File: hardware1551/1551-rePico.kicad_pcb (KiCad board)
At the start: 2 copper layers, 59.1 x 60 mm, 44 parts, among them IC1 VIA6522, J1 Display Connector, J2 Display Power, J3 Conn_01x05_Pin, J4 SD Card Module Connector, J5 Conn_01x01_Pin, J6 EXT_5V, J7 RESET_1541, P1 VIA_PIN_1-20, P2 VIA_PIN_21-40, Q1 BSS138, Q2 BSS138, Q3 BSS138, Q4 BSS138, Q5 BSS138, Q6 BSS138, Q7 BSS138, Q8 BSS138, Q9 BSS138, SW1 RESET, U1 Pico, U2 SN74LVC4245A

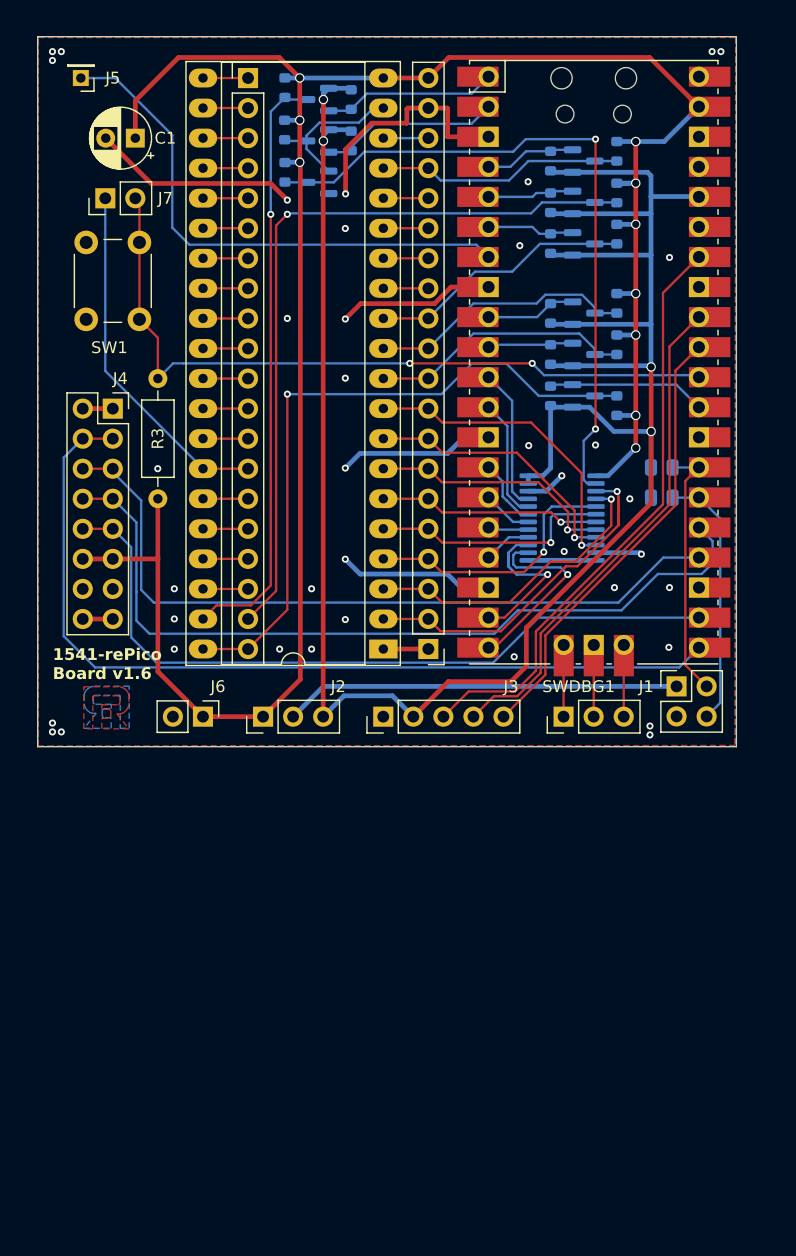
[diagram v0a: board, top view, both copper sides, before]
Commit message: updated
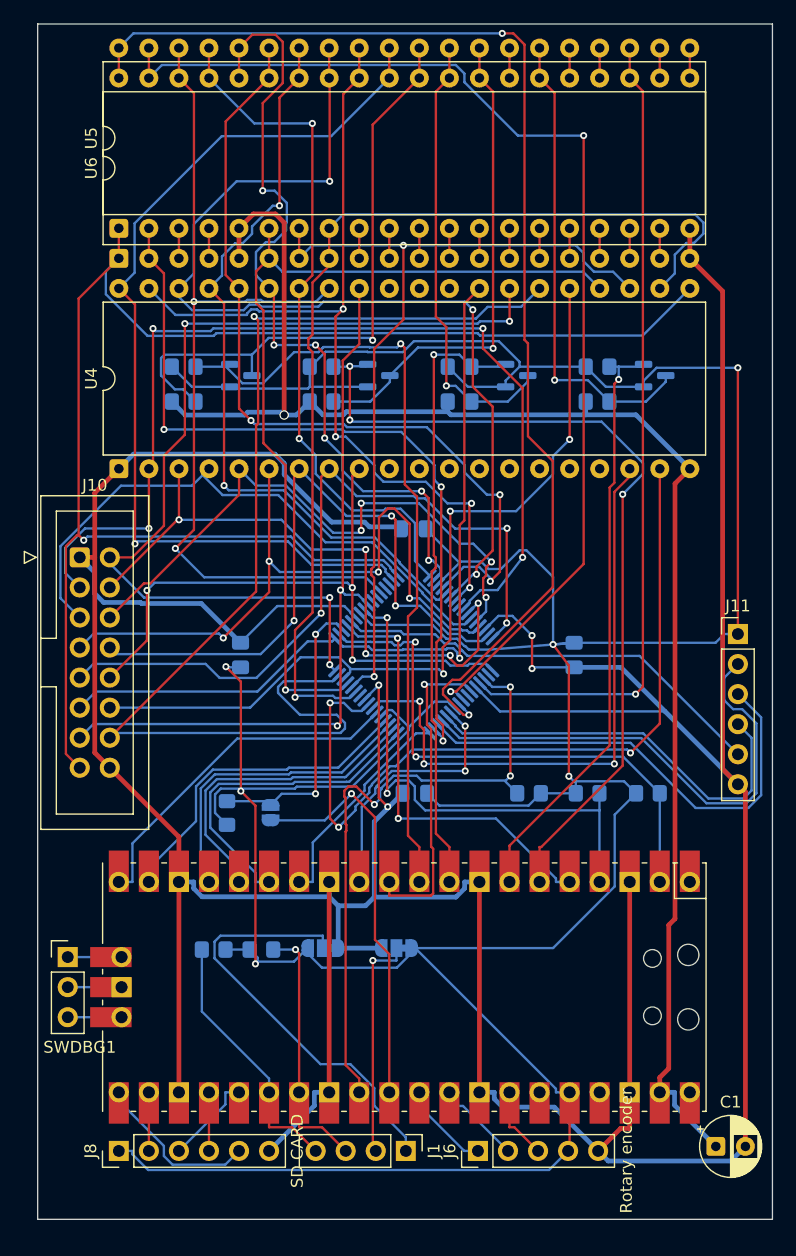
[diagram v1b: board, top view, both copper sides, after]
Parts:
- removed IC1: VIA6522, Package_DIP:DIP-40_W15.24mm_Socket_LongPads
- removed J2: Display Power, Connector_PinHeader_2.54mm:PinHeader_1x03_P2.54mm_Vertical
- removed J3: Conn_01x05_Pin, Connector_PinHeader_2.54mm:PinHeader_1x05_P2.54mm_Vertical
- removed J4: SD Card Module Connector, Connector_PinSocket_2.54mm:PinSocket_2x08_P2.54mm_Vertical
- removed J5: Conn_01x01_Pin, Connector_PinHeader_2.00mm:PinHeader_1x01_P2.00mm_Vertical
- removed J7: RESET_1541, Connector_PinHeader_2.54mm:PinHeader_1x02_P2.54mm_Vertical
- removed P1: VIA_PIN_1-20, Connector_PinHeader_2.54mm:PinHeader_1x20_P2.54mm_Vertical
- removed P2: VIA_PIN_21-40, Connector_PinHeader_2.54mm:PinHeader_1x20_P2.54mm_Vertical
- removed Q5, Q6, Q7, Q8, Q9: BSS138, Package_TO_SOT_SMD:SOT-23
- removed R15, R16, R17, R18, R19, R20: 10k, Resistor_SMD:R_0603_1608Metric
- removed SW1: RESET, Button_Switch_THT:SW_PUSH_6mm_H5mm
- removed U2: SN74LVC4245A, Package_SO:TSSOP-24_4.4x7.8mm_P0.65mm
- added C2: 0.1uF, Capacitor_SMD:C_0805_2012Metric_Pad1.18x1.45mm_HandSolder, B.Cu at (117.3, 117.3)
- added C3: 0.1uF, Capacitor_SMD:C_0805_2012Metric_Pad1.18x1.45mm_HandSolder, B.Cu at (145.5, 117.3)
- added C4: 0.1uF, Capacitor_SMD:C_0805_2012Metric_Pad1.18x1.45mm_HandSolder, B.Cu at (132.1, 129.0)
- added C5: 0.1uF, Capacitor_SMD:C_0805_2012Metric_Pad1.18x1.45mm_HandSolder, B.Cu at (131.9, 106.7)
- added J10: TCBM, Connector_IDC:IDC-Header_2x08_P2.54mm_Vertical, F.Cu at (103.7, 109.1)
- added J11: JTAG, Connector_PinHeader_2.54mm:PinHeader_1x06_P2.54mm_Vertical, F.Cu at (159.4, 115.5)
- added J8: SD CARD, Connector_PinHeader_2.54mm:PinHeader_1x06_P2.54mm_Vertical, F.Cu at (107.0, 159.2)
- added JP1: ~, Jumper:SolderJumper-2_P1.3mm_Open_RoundedPad1.0x1.5mm, B.Cu at (119.9, 130.6)
- added JP3: SolderJumper_3_Bridged12, Jumper:SolderJumper-3_P1.3mm_Bridged12_RoundedPad1.0x1.5mm_NumberLabels, B.Cu at (124.3, 142.1)
- added JP4: SolderJumper_3_Bridged12, Jumper:SolderJumper-3_P1.3mm_Bridged12_RoundedPad1.0x1.5mm_NumberLabels, B.Cu at (130.5, 142.1)
- added U3: XC9572XL-VQ64, Package_QFP:TQFP-64_10x10mm_P0.5mm, B.Cu at (132.0, 117.3)
- added U4: 6523 (pins), Package_DIP:DIP-40_W15.24mm, F.Cu at (107.0, 101.6)
- added U5: 6510T (pins), Package_DIP:DIP-40_W15.24mm, F.Cu at (107.0, 81.3)
- added U6: 6510T (socket for chip), Package_DIP:DIP-40_W15.24mm, F.Cu at (107.0, 83.8)
- J1: value Display Connector -> 0.96_I2C_OLED; footprint Connector_PinSocket_2.54mm:PinSocket_2x02_P2.54mm_Vertical -> Connector_PinHeader_2.54mm:PinHeader_1x04_P2.54mm_Vertical
- J6: value EXT_5V -> Rotary encoder; footprint Connector_PinHeader_2.54mm:PinHeader_1x02_P2.54mm_Vertical -> Connector_PinHeader_2.54mm:PinHeader_1x05_P2.54mm_Vertical
- R1, R2: value 1.8k -> 10k; footprint Resistor_SMD:R_0805_2012Metric -> Resistor_SMD:R_0805_2012Metric_Pad1.20x1.40mm_HandSolder
- R10, R11, R12, R13, R14, R5, R6, R7, R8, R9: footprint Resistor_SMD:R_0603_1608Metric -> Resistor_SMD:R_0805_2012Metric_Pad1.20x1.40mm_HandSolder
- R3: footprint Resistor_THT:R_Axial_DIN0207_L6.3mm_D2.5mm_P10.16mm_Horizontal -> Resistor_SMD:R_0805_2012Metric_Pad1.20x1.40mm_HandSolder; moved to B.Cu
- R4: value 1M -> 10k; footprint Resistor_SMD:R_0603_1608Metric -> Resistor_SMD:R_0805_2012Metric_Pad1.20x1.40mm_HandSolder
- moved C1 98.3 mm to (157.5, 158.9), turned to 0 degrees
- moved R14 69.5 mm to (115.1, 142.2), turned to 180 degrees
- moved R13 68.8 mm to (119.1, 142.2), turned to 0 degrees
- moved U1 55.2 mm to (131.2, 145.4), turned to -90 degrees
- moved R12 54.3 mm to (146.7, 129.0), turned to 0 degrees
- moved R11 54.1 mm to (151.8, 129.0), turned to 0 degrees
- moved R7 50.3 mm to (116.2, 130.7)
- moved SWDBG1 46.6 mm to (102.7, 142.8), turned to 0 degrees
- moved J1 45.4 mm to (131.3, 159.2), turned to -90 degrees
- moved J6 43.4 mm to (137.4, 159.2), turned to 90 degrees
- moved R8 42.1 mm to (141.7, 129.0), turned to 180 degrees
- moved R6 36.9 mm to (112.5, 95.9), turned to 0 degrees
- moved R5 31.0 mm to (112.5, 93.0), turned to 0 degrees
- moved R1 30.0 mm to (124.2, 93.0)
- moved R2 29.9 mm to (124.2, 95.9)
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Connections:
- net /VIA 6522 Sockel/MTR renamed /WPS
- J1 pad 2: GND -> Net-(J1-Pin_2)
- J1 pad 3: I2C_SCL -> /I2C_SCL
- J1 pad 4: I2C_SDA -> /I2C_SDA
- J6 pad 1: +5V -> /ROT_CLK
- J6 pad 2: GND -> /ROT_DT
- Q1 pad 1: /VIA 6522 Sockel/MODE -> +3V3
- Q1 pad 2: GND -> /MTR_3V3
- Q1 pad 3: Net-(Q1-D) -> /MTR
- Q2 pad 1: +3.3V -> +3V3
- Q2 pad 2: /_STP1 -> /STP0_3V3
- Q2 pad 3: /VIA 6522 Sockel/STP1 -> /STP0
- Q3 pad 1: +3.3V -> +3V3
- Q3 pad 2: /_STP0 -> /STP1_3V3
- Q3 pad 3: /VIA 6522 Sockel/STP0 -> /STP1
- Q4 pad 1: +3.3V -> +3V3
- Q4 pad 2: /_MTR -> /WPS_3V3
- R1 pad 1: +3.3V -> +3V3
- R1 pad 2: I2C_SCL -> /MTR_3V3
- R11 pad 1: +3.3V -> +3V3
- R11 pad 2: /_SYNC -> /MODE_3V3
- R12 pad 1: +5V -> +3V3
- R12 pad 2: /VIA 6522 Sockel/SYNC -> /SYNC_3V3
- R13 pad 1: +3.3V -> +3V3
- R13 pad 2: /_OE -> /I2C_SCL
- R14 pad 1: +5V -> +3V3
- R14 pad 2: /VIA 6522 Sockel/MODE -> /I2C_SDA
- R2 pad 1: +3.3V -> +5V
- R2 pad 2: I2C_SDA -> /MTR
- R3 pad 1: Net-(J7-Pin_2) -> +3V3
- R3 pad 2: +5V -> /STP0_3V3
- R4 pad 2: Net-(Q1-D) -> /STP0
- R5 pad 1: +3.3V -> +3V3
- R5 pad 2: /_STP1 -> /STP1_3V3
- R6 pad 2: /VIA 6522 Sockel/STP1 -> /STP1
- R7 pad 1: +3.3V -> +3V3
- R7 pad 2: /_STP0 -> /~{RESET_3V3}
- R8 pad 1: +5V -> +3V3
- R8 pad 2: /VIA 6522 Sockel/STP0 -> /BYTE_READY_3V3
- R9 pad 1: +3.3V -> +3V3
- R9 pad 2: /_MTR -> /WPS_3V3
- U1 pad 1: /_SOE -> unconnected-(U1-GPIO0-Pad1)
- U1 pad 10: /_STP1 -> /STP1_3V3
- U1 pad 11: /_PA0 -> /YB0
- U1 pad 12: /_PA1 -> /YB1
- U1 pad 14: /_PA2 -> /YB2
- U1 pad 15: /_PA3 -> /YB3
- U1 pad 16: /_PA4 -> /YB4
- U1 pad 17: /_PA5 -> /YB5
- U1 pad 19: /_PA6 -> /YB6
- U1 pad 2: /_OE -> /MODE_3V3
- U1 pad 20: /_PA7 -> /YB7
- U1 pad 21: MISO -> /SD_MISO
- U1 pad 22: CS -> /SD_CS
- U1 pad 24: SCK -> /SD_SCK
- U1 pad 25: MOSI -> /SD_MOSI
- U1 pad 26: I2C_SDA -> /I2C_SDA
- U1 pad 27: I2C_SCL -> /I2C_SCL
- U1 pad 29: /_BRDY -> /BYTE_READY_3V3
- U1 pad 30: Net-(J7-Pin_2) -> Net-(JP1-B)
- U1 pad 31: Net-(J3-Pin_5) -> /ROT_CLK
- U1 pad 32: Net-(J3-Pin_4) -> /ROT_DT
- U1 pad 33: unconnected-(U1-AGND-Pad33)_1 -> GND
- U1 pad 34: Net-(J3-Pin_3) -> /ROT_SW
- U1 pad 36: +3.3V -> +3V3
- U1 pad 4: /_SYNC -> /SYNC_3V3
- U1 pad 5: /_SOE_GA -> /DEVNUM_3V3
- U1 pad 6: /_MTR -> /MTR_3V3
- U1 pad 7: Net-(J5-Pin_1) -> /WPS_3V3
- U1 pad 9: /_STP0 -> /STP0_3V3
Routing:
- net +3V3: track 0.00 -> 346.3 mm, vias 0 -> 6
- net GND: track 99.7 -> 392.0 mm, vias 39 -> 4
- net +3.3V: track 194.6 -> 0.00 mm, vias 4 -> 0
- net /~{RESET}: track 0.00 -> 132.9 mm, vias 0 -> 1
- net /PHI2: track 0.00 -> 102.0 mm, vias 0 -> 2
- net /STATUS1: track 0.00 -> 99.7 mm, vias 0 -> 1
- net /R/~{W}: track 0.00 -> 95.9 mm, vias 0 -> 2
- net /A2: track 0.00 -> 86.5 mm, vias 0 -> 1
- net /DIO1: track 0.00 -> 84.6 mm, vias 0 -> 4
- net /D5: track 0.00 -> 83.5 mm, vias 0 -> 3
- net /D7: track 0.00 -> 80.8 mm, vias 0 -> 1
- net /DEV: track 0.00 -> 80.4 mm, vias 0 -> 4
- net MISO: track 75.4 -> 0.00 mm
- net /A0: track 0.00 -> 75.0 mm, vias 0 -> 1
- net /D6: track 0.00 -> 74.6 mm, vias 0 -> 4
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- removed copper zone on B.Cu, net (none)
- removed copper zone on F.Cu, net (none)
- removed copper zone on B.Cu, net GND
- removed copper zone on F.Cu, net GND
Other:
- board size 59.1 x 60 mm -> 62.1 x 101 mm
- board text removed: "1541-rePico Board v1.6"
- board text removed: "https://github.com/fook42/1541-rePico"
